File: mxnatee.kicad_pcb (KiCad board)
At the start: 2 copper layers, 128.3 x 129.4 mm, 43 parts, among them U1 ProMicro, U2 TRRS

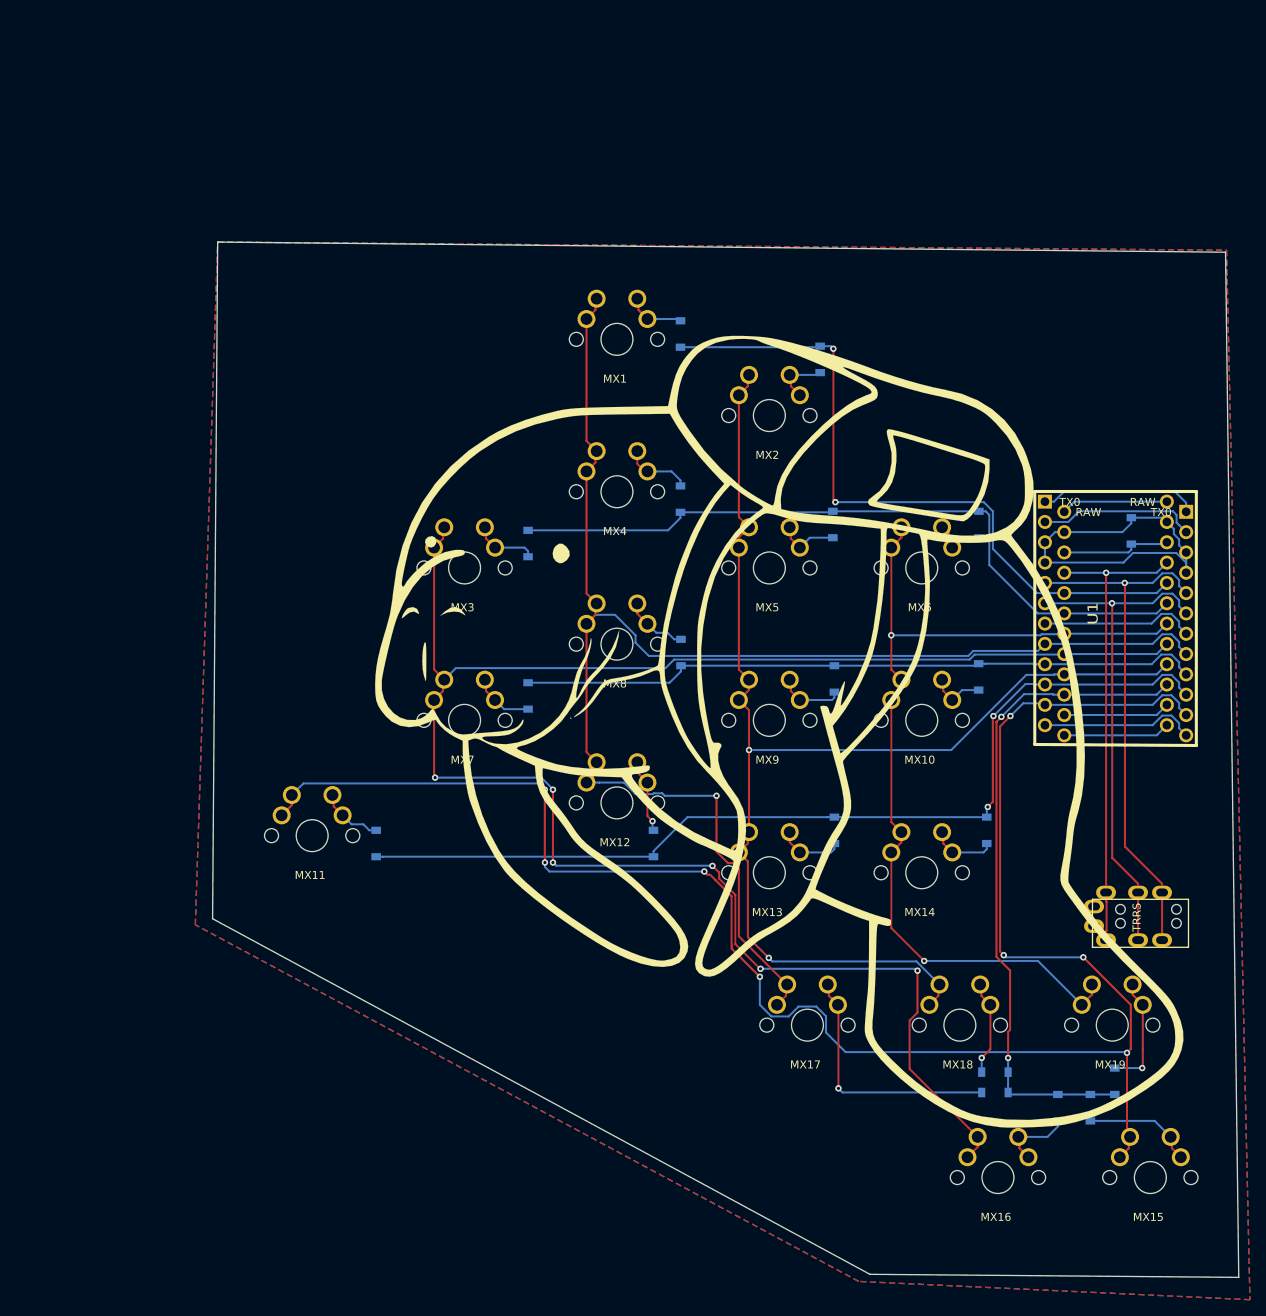
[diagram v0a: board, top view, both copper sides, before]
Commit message: Initial attempt at doing cool edge cuts
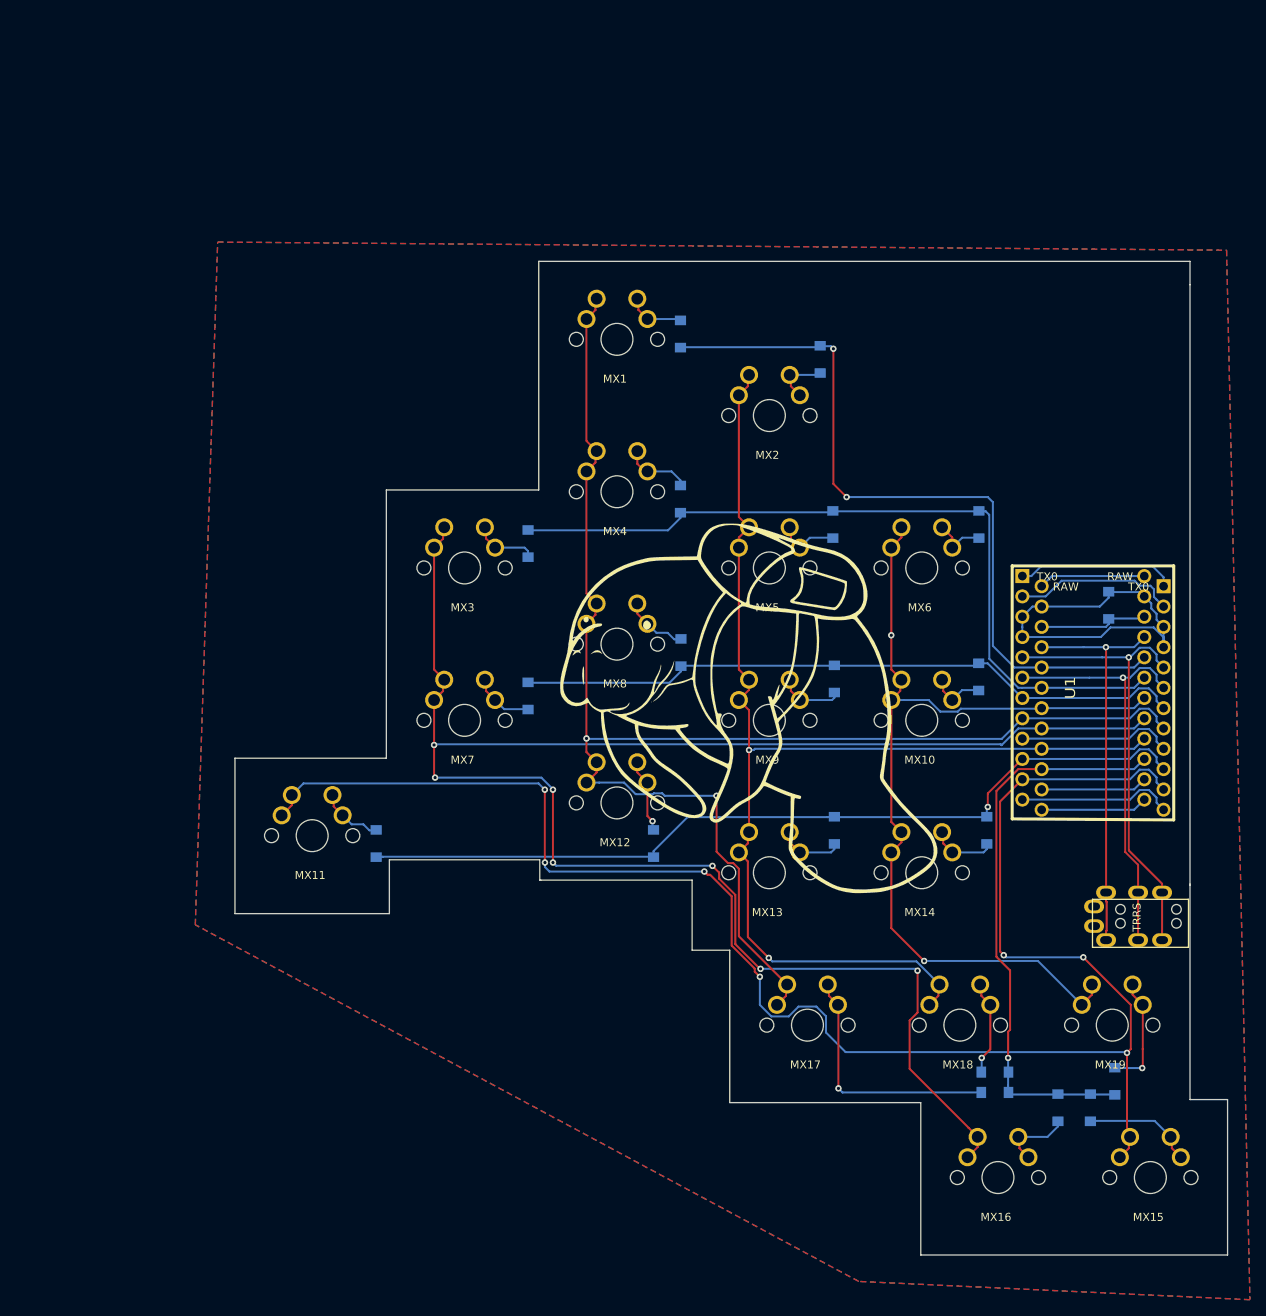
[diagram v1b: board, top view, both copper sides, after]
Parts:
- removed the G*** at (104.8, 102.5) (x2)
- added G***: LOGO, SILK:mxnatee, F.Cu at (100.2, 98.7)
- D1, D10, D11, D12, D13, D14, D15, D16, D17, D18, D19, D2, D21, D3, D4, D5, D6, D7, D8, D9: footprint random-keyboard-parts:D_SOD-123-Pretty -> Keebio-Parts:D_SOD123
- moved D21 9.72 mm to (144.5, 85.0)
- moved U1 9.72 mm to (141.4, 95.3)
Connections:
- U1 pad 7: Net-(U1-Pad7) -> ROW2
- U1 pad 9: ROW2 -> Net-(U1-Pad9)
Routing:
- net Net-(U1-Pad7): track 20.2 -> 0.00 mm
- net Net-(U1-Pad9): track 0.00 -> 19.7 mm
- net COL0: track 229.4 -> 217.3 mm, vias 8 -> 7
- net ROW3: track 119.4 -> 107.4 mm, vias 2 -> 1
- net ROW4: track 83.9 -> 72.1 mm, vias 2 -> 1
- net DATA1: track 63.1 -> 53.2 mm
- net DATA2: track 66.4 -> 56.7 mm
- net VCC: track 59.3 -> 50.0 mm
- net ROW1: track 90.9 -> 98.8 mm
- net ROW0: track 88.0 -> 95.6 mm
- net COL3: track 160.6 -> 153.9 mm
- net COL2: track 192.9 -> 187.4 mm, vias 1 -> 2
- net COL4: track 119.4 -> 117.3 mm
- net COL1: track 232.6 -> 230.8 mm, vias 6 -> 7
- net ROW2: track 85.8 -> 85.2 mm
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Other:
- board size 128.3 x 129.4 mm -> 124.1 x 124.2 mm

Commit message: Rev 1
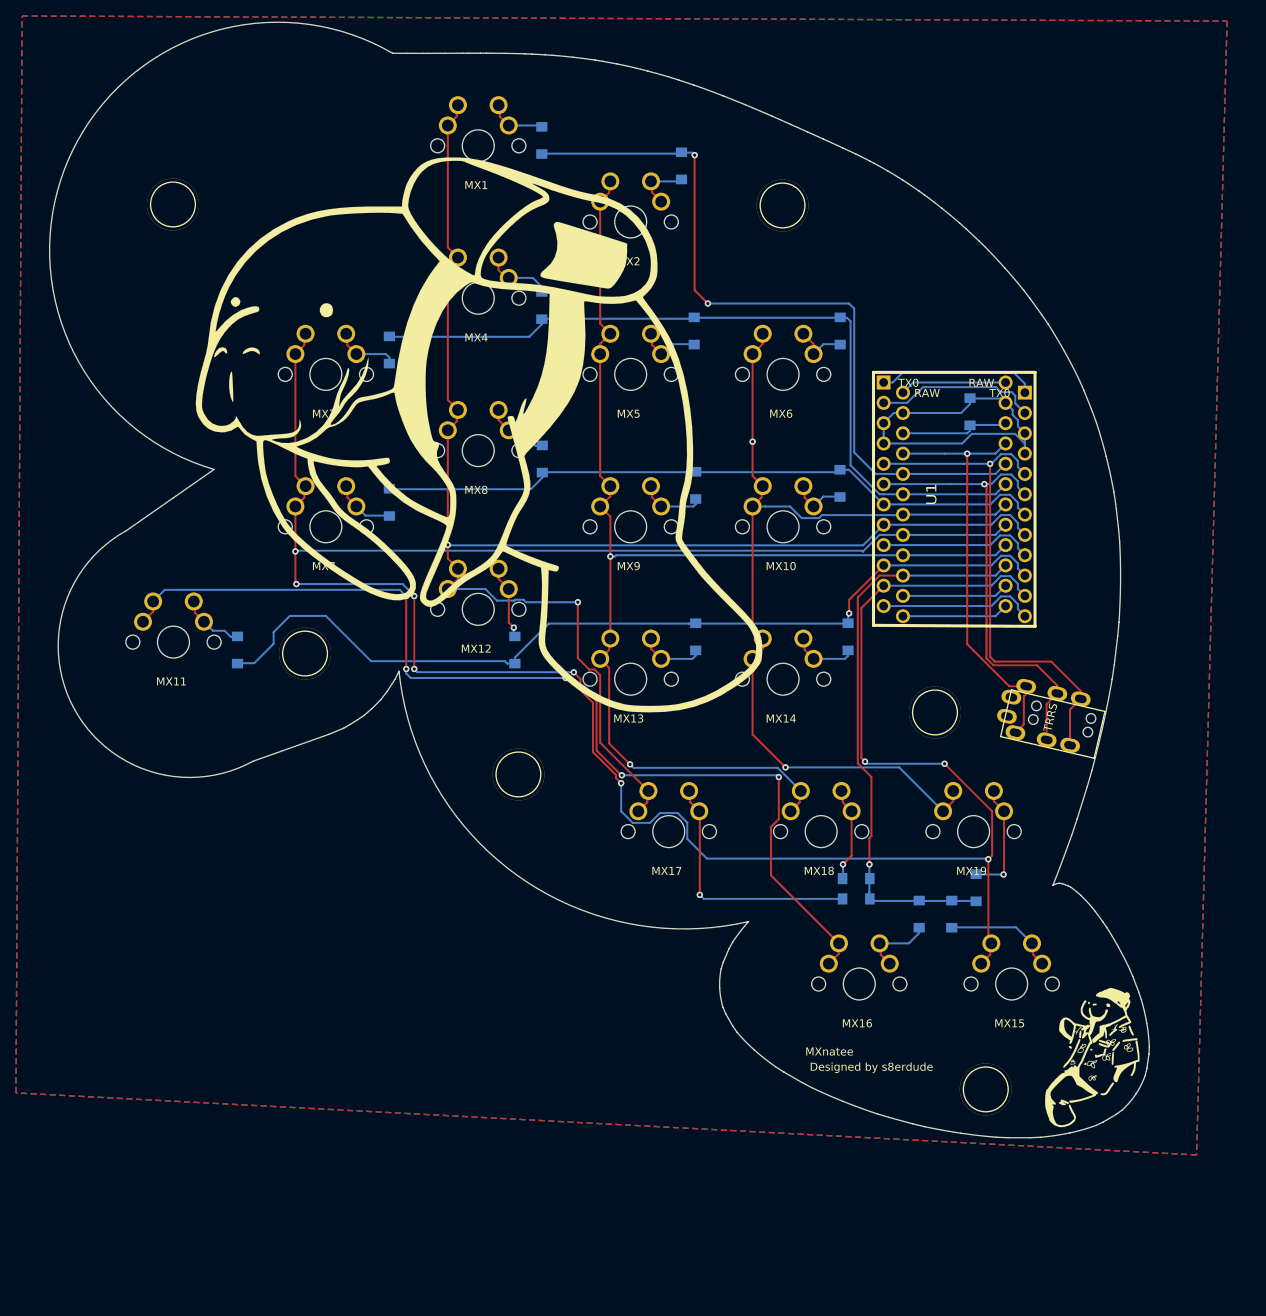
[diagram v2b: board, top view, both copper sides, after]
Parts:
- removed the G*** at (100.2, 98.7)
- added G***: LOGO, SILK:mxnatee_med, F.Cu at (66.9, 64.9)
- added G***: LOGO, SILK:mxnatee_med_back, B.Cu at (66.9, 65.0)
- added G***: LOGO, SILK:me, F.Cu at (142.4, 141.2)
- added U4: HOLE, Keebio-Parts:MountingHole, F.Cu at (103.8, 35.1)
- added U4: HOLE, Keebio-Parts:MountingHole, F.Cu at (122.8, 98.4)
- added U4: HOLE, Keebio-Parts:MountingHole, F.Cu at (129.2, 145.5)
- added U4: HOLE, Keebio-Parts:MountingHole, F.Cu at (70.7, 106.2)
- added U4: HOLE, Keebio-Parts:MountingHole, F.Cu at (44.1, 91.1)
- added U4: HOLE, Keebio-Parts:MountingHole, F.Cu at (27.6, 34.9)
- moved D19 29.8 mm to (128.0, 120.3)
- moved D5 29.8 mm to (92.7, 50.7)
- moved MX1 29.8 mm to (65.7, 27.7)
- moved MX4 29.8 mm to (65.7, 46.8)
- moved D1 29.8 mm to (73.7, 26.9)
- moved D10 29.8 mm to (110.9, 69.8)
- moved D13 29.8 mm to (92.9, 89.0)
- moved D15 29.8 mm to (124.9, 123.6)
- moved D18 29.8 mm to (113.0, 119.2)
- moved D21 29.8 mm to (127.2, 60.8)
- moved D9 29.8 mm to (92.9, 70.0)
- moved MX12 29.8 mm to (65.7, 85.7)
- moved MX13 29.8 mm to (84.8, 94.4)
- moved MX2 29.8 mm to (84.8, 37.2)
- moved MX5 29.8 mm to (84.8, 56.3)
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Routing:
- net DATA2: track 56.7 -> 64.2 mm
- net DATA1: track 53.2 -> 59.1 mm
- net ROW3: track 107.4 -> 113.2 mm
- net VCC: track 50.0 -> 53.1 mm
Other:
- board size 124.1 x 124.2 mm -> 137.5 x 139.4 mm
- board text added: "Designed by s8erdude"
- board text added: "MXnatee"
